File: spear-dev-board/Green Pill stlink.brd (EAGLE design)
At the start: 53.2 x 21 mm, 41 parts, among them IC1 STM32F103C8T6, IC2 STM32F103C8T6, U1 3.3V, X1 8MHz, X2 8MHz

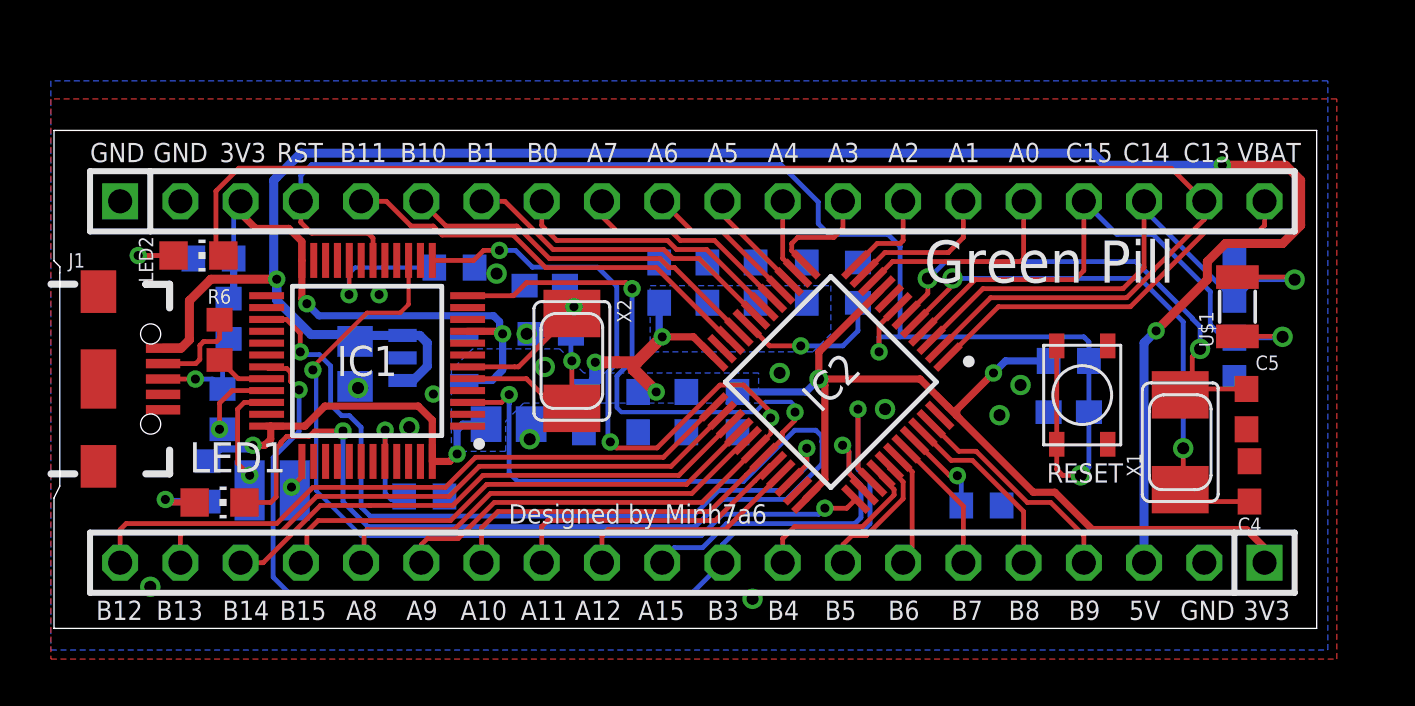
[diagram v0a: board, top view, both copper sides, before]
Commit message: added jumper for MCO switch, updated design
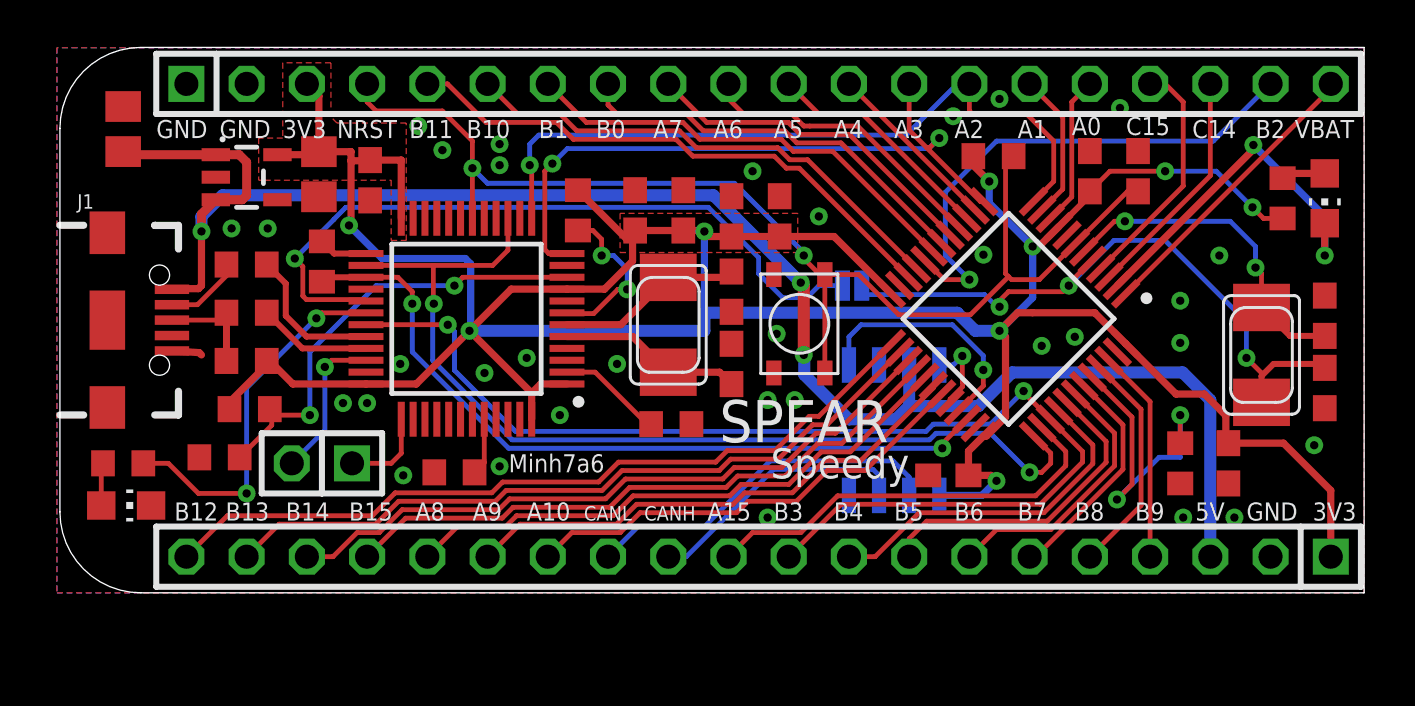
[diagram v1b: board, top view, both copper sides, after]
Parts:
- removed C6, C7: 22pF, resistor:C0603
- removed DCLK, DIO: (no value), wirepad:SMD1,27-2,54
- added JP3: (no value), pinhead:1X02
- added R11, R12: 4.7k, rcl:R0603
- added R13: 1k, rcl:R0603
- added SJ1: SOLDERJUMPERNC2, SparkFun-Retired:SJ_2S-NOTRACE
- R1, R3: value 10k -> 100k
- R7: value 10k -> 1.5k
- R9: value 1k -> 100
- U$1: value 32.768kHz -> MCP2562-E/SN; device SPEAR:3.2X1.5 -> SPEAR:SOIC8
- moved LED2 47.6 mm to (53.3, 16.6), turned to 180 degrees
- moved R10 45.2 mm to (51.6, 16.6), flipped to the top, turned to 90 degrees
- moved C14 23.0 mm to (49.3, 5.46), flipped to the top
- moved C16 18.8 mm to (43.4, 17.8), flipped to the top
- moved U$1 15.4 mm to (35.2, 6.86), flipped to the bottom, turned to 180 degrees
- moved C17 14.9 mm to (13.1, 17.4), flipped to the top, turned to 270 degrees
- moved C1 13.9 mm to (2.67, 19.6), flipped to the top, turned to 90 degrees
- moved C13 13.4 mm to (37.5, 4.95), flipped to the top, turned to 180 degrees
- moved C2 13.2 mm to (10.9, 17.7), flipped to the top, turned to 270 degrees
- moved U1 11.0 mm to (7.87, 17.5), flipped to the top, turned to 270 degrees
- moved C10 10.6 mm to (45.5, 17.8), flipped to the top, turned to 90 degrees
- moved R9 10.5 mm to (11.0, 14.0), flipped to the top, turned to 270 degrees
- moved R2 9.88 mm to (25.8, 7.11), flipped to the top, turned to 0 degrees
- moved U$2 9.85 mm to (32.3, 9.27), turned to 90 degrees
- moved R8 9.20 mm to (39.4, 18.4), flipped to the top, turned to 180 degrees
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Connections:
- new net CANH: JP1.12, U$1.7
- new net CANL: JP1.13, U$1.6
- new net LED_STLINK: IC1.30, R13.1
- new net N$10: IC1.29, SJ1.1
- new net PA0: IC1.10, R11.1, R12.2
- new net RST: IC1.7, R4.1
- net 3.3V: now also IC1.1, R11.2, R4.2, U$1.5; no longer R9.2
- net 5V: now also U$1.3
- net DCLK: now also JP3.1; no longer DCLK.1
- net DIO: now also JP3.2; no longer DIO.1
- net GND: now also IC1.20, LED1.C, R12.1, U$1.2, U$1.8; no longer C6.2, C7.2, R4.2
- net N$5: now also IC1.2, R2.1; no longer IC1.20, R4.1
- net N$7: now also LED1.A, R13.2; no longer IC1.3, LED1.C
- net N$8: now also IC1.25; no longer LED1.A
- net OSC32_IN: no longer C7.1, U$1.2
- net OSC32_OUT: no longer C6.1, U$1.1
- net OSC_IN: now also SJ1.2
- net PA10: no longer IC1.12
- net PA11: now also U$1.4; no longer JP1.13
- net PA12: now also U$1.1; no longer JP1.12
- net PA2: now also IC1.13
- net PA3: now also IC1.12
- net PA9: no longer IC1.13
- net PB2: now also JP2.19; no longer R2.1
- net PC13: no longer JP2.19
- net SWCLK: now also IC1.26
- net SWDIO: now also R9.2
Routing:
- net 3.3V: track 93.2 -> 146.8 mm
- net N$7: track 52.1 -> 1.81 mm, vias 2 -> 0
- net PC13: track 59.8 -> 15.6 mm, vias 0 -> 2
- net N$10: track 0.00 -> 30.6 mm, vias 0 -> 1
- net PA2: track 4.07 -> 30.9 mm, vias 0 -> 1
- net PA3: track 4.71 -> 28.6 mm, vias 0 -> 2
- net PA9: track 42.1 -> 21.8 mm, vias 3 -> 0
- net PA0: track 0.00 -> 19.1 mm, vias 0 -> 2
- net PA10: track 37.7 -> 19.5 mm, vias 2 -> 0
- net LED_STLINK: track 0.00 -> 15.7 mm, vias 0 -> 2
- net CANL: track 0.00 -> 15.4 mm
- net PB2: track 6.51 -> 21.9 mm
- net 5V: track 87.2 -> 72.7 mm
- net OSC32_IN: track 24.1 -> 9.92 mm, vias 1 -> 0
- net OSC32_OUT: track 24.3 -> 10.2 mm, vias 1 -> 0
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- added copper zone on layer 1, net 3.3V
- removed copper zone on layer 16, net 3.3V
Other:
- board size 53.2 x 21 mm -> 55 x 23 mm
- board text added: "B2"
- board text added: "CANH"
- board text added: "CANL"
- board text added: "Minh7a6"
- board text added: "NRST"
- board text added: "SPEAR"
- board text added: "Speedy"
- board text removed: "A11"
- board text removed: "A12"
- board text removed: "C13"
- board text removed: "Designed by Minh7a6"
- board text removed: "Green Pill"
- board text removed: "RESET"
- board text removed: "RST"
